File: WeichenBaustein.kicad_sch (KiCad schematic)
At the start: 8 parts, among them J1 Conn_01x16, J7 Conn_01x12_Female, U2 esp32_dev4_left, U3 esp32_dev4_right

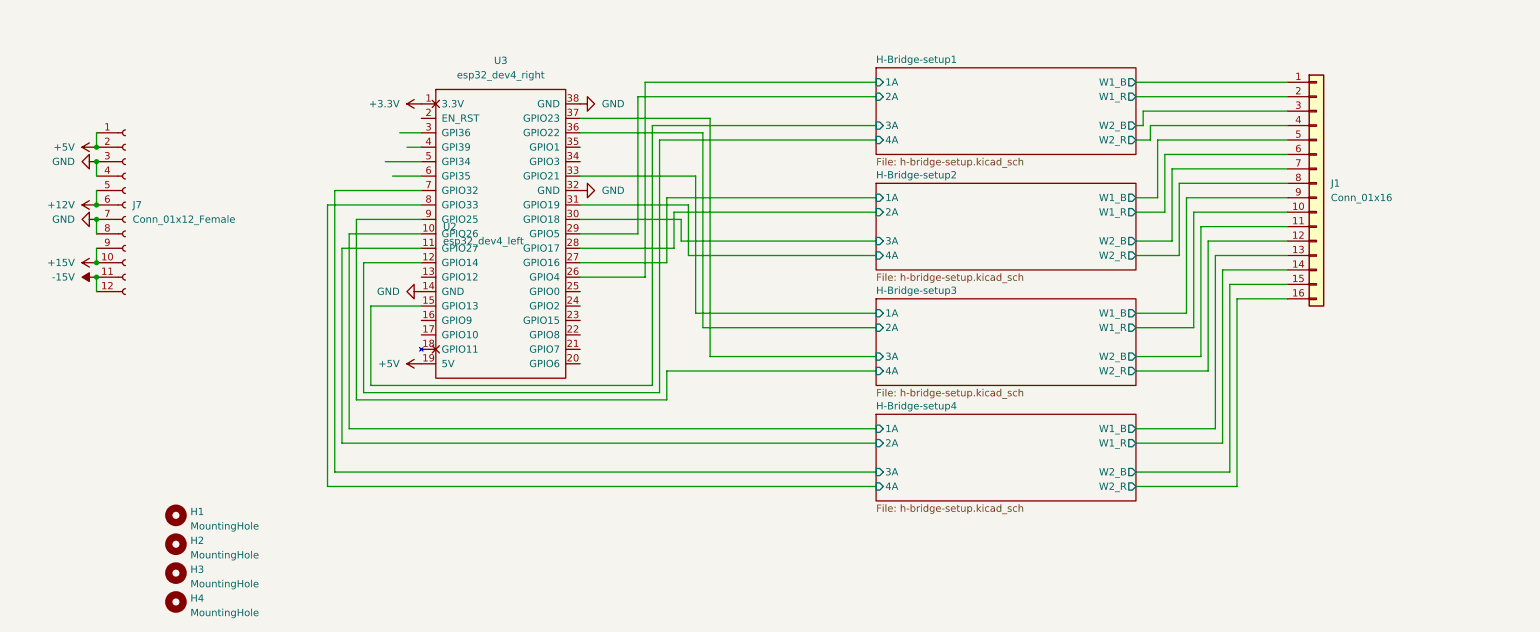
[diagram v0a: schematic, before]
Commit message: scematics and basic PCB layout
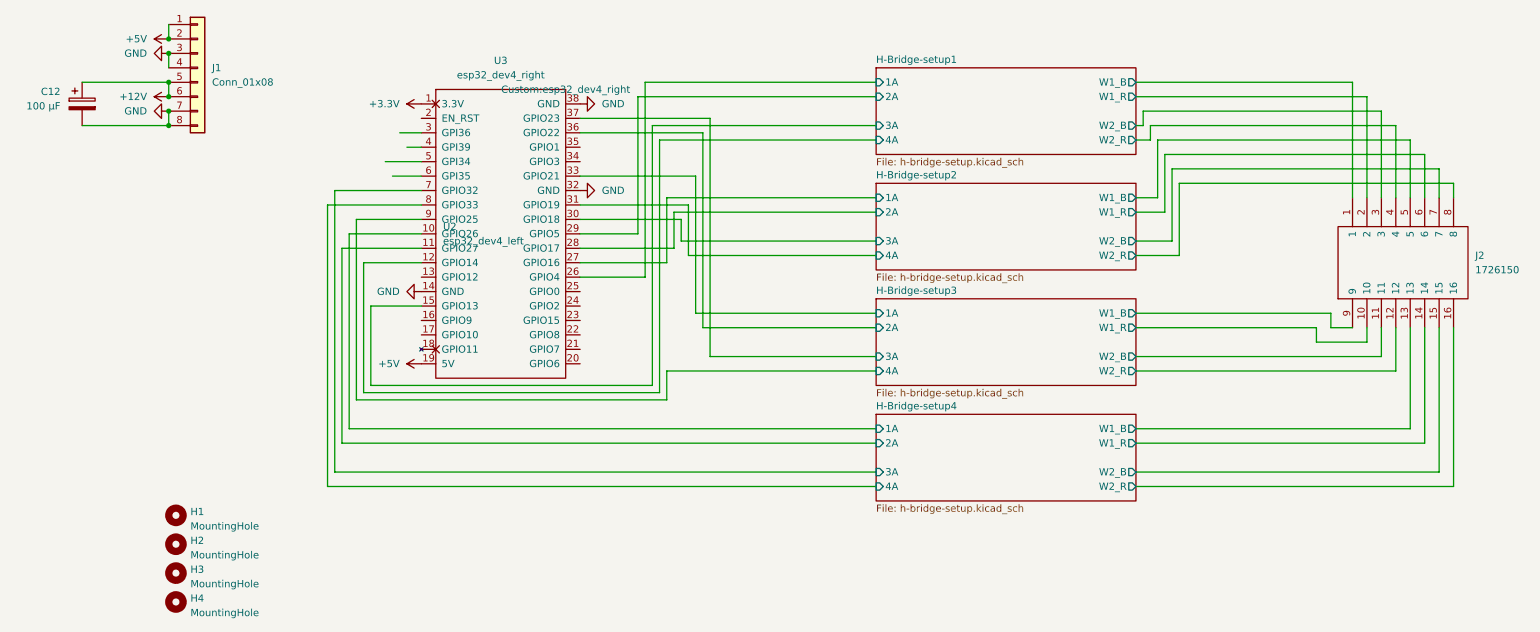
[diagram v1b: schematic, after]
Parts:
- removed J1: Conn_01x16, symbol Connector_Generic:Conn_01x16
- removed J7: Conn_01x12_Female, Custom:1729225, symbol Connector:Conn_01x12_Female
- added C12: 100 µF, Capacitor_THT:CP_Radial_D6.3mm_P2.50mm, symbol Device:C_Polarized
- added J1: Conn_01x08, Custom:1729186, symbol Connector_Generic:Conn_01x08
- added J2: 1726150, 1726150, symbol Custom:1726150
- U2: footprint fp_esp32_dev4:esp32_dev_left -> Custom:esp32_dev_left
- U3: footprint fp_esp32_dev4:esp32_dev4_right -> Custom:esp32_dev4_right
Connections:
- net +12V: now also C12.1, J1.5 (Pin_5), J1.6 (Pin_6)
- net +5V: now also J1.1 (Pin_1), J1.2 (Pin_2)
- net GND: now also C12.2, J1.3 (Pin_3), J1.4 (Pin_4), J1.7 (Pin_7), J1.8 (Pin_8)
- net H-Bridge-setup1/W1_B: now also J2.1
- net H-Bridge-setup1/W1_R: now also J2.2
- net H-Bridge-setup1/W2_B: now also J2.3
- net H-Bridge-setup1/W2_R: now also J2.4
- net H-Bridge-setup2/W1_B: now also J2.5
- net H-Bridge-setup2/W1_R: now also J2.6
- net H-Bridge-setup2/W2_B: now also J2.7
- net H-Bridge-setup2/W2_R: now also J2.8
- net H-Bridge-setup3/W1_B: now also J2.9
- net H-Bridge-setup3/W1_R: now also J2.10
- net H-Bridge-setup3/W2_B: now also J2.11
- net H-Bridge-setup3/W2_R: now also J2.12
- net H-Bridge-setup4/W1_B: now also J2.13
- net H-Bridge-setup4/W1_R: now also J2.14
- net H-Bridge-setup4/W2_B: now also J2.15
- net H-Bridge-setup4/W2_R: now also J2.16
